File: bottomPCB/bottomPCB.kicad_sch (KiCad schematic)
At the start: 20 parts, among them P1 Pfostenstecker_8_2x4, U1 ESP32-WROOM-32, U2 Pfostenstecker_6_2x3, U3 Switch

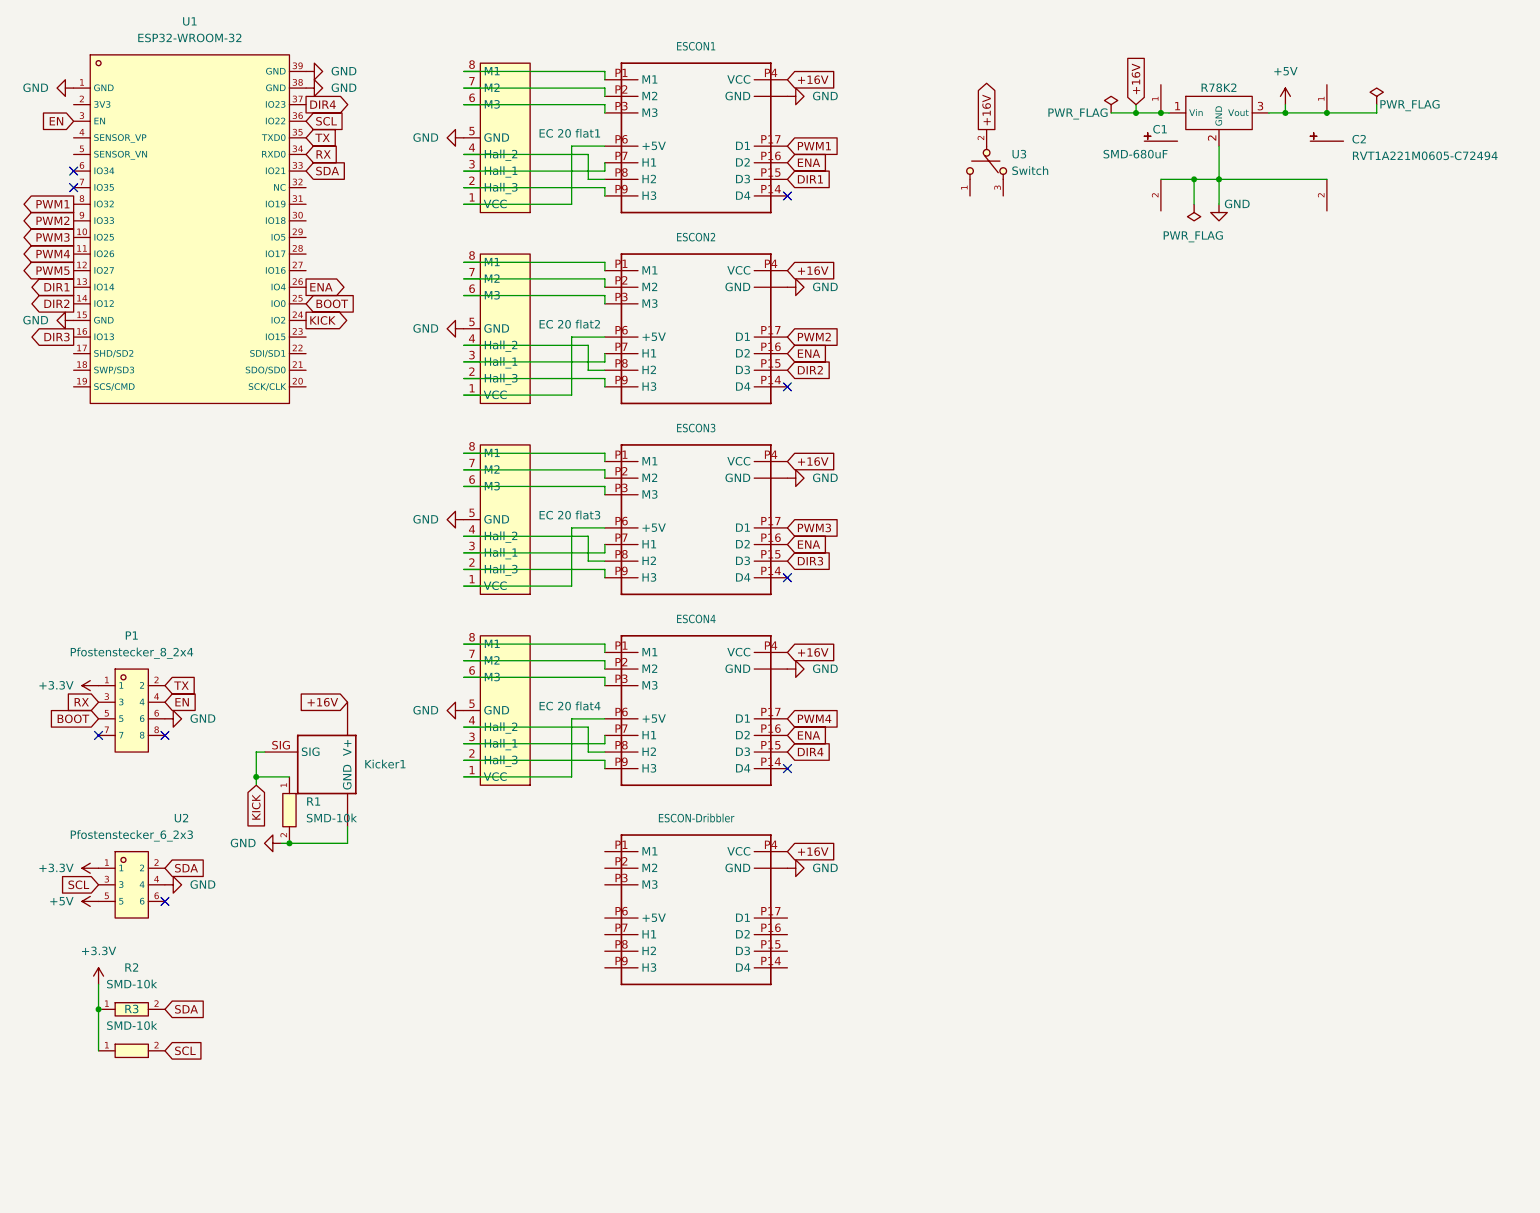
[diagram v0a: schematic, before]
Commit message: lichtschranke
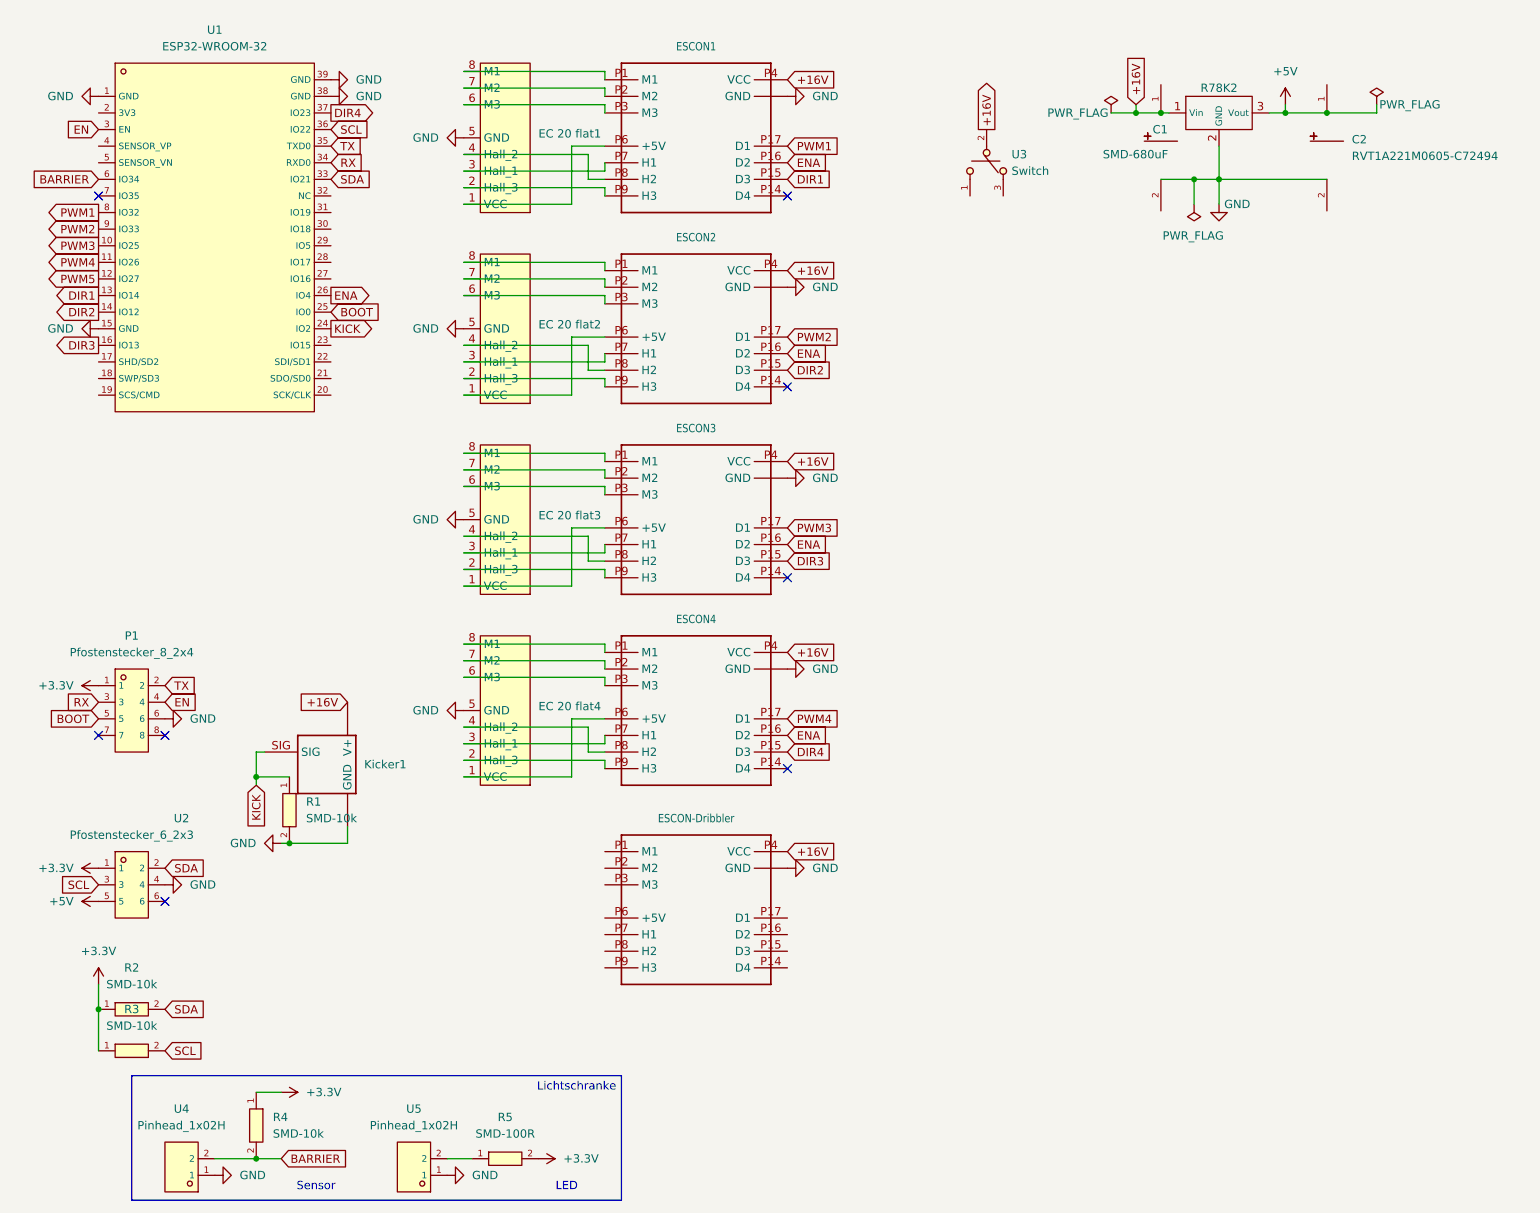
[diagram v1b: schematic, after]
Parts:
- added R4: SMD-10k, BohleBots:R0603, symbol bohlebots.lib:SMD-10k
- added R5: SMD-100R, BohleBots:R0603, symbol bohlebots.lib:SMD-100R
- added U4, U5: Pinhead_1x02H, BohleBots:HDR-TH_2P-P2.54-H-M-W10.4, symbol bohlebots.lib:Pinhead_1x02H
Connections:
- net +3.3V: now also R4.1, R5.2
- net GND: now also U4.1, U5.1
- net BARRIER: now reaches U1.6 (IO34)
- net BARRIER: now also R4.2, U4.2
- new net: R5.1, U5.2
- no-connect marks 9 -> 8
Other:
- note added: "LED"
- note added: "Lichtschranke"
- note added: "Sensor"
- moved on the sheet: U1
